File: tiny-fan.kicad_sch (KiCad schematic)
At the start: 41 parts, among them Q1 BSS138, Q2 BSS138, Q3 BSS138, Q4 BSS138, Q5 BSS138, Q6 BSS138, Q7 BSS138, U1 L7812, U2 tiny2040

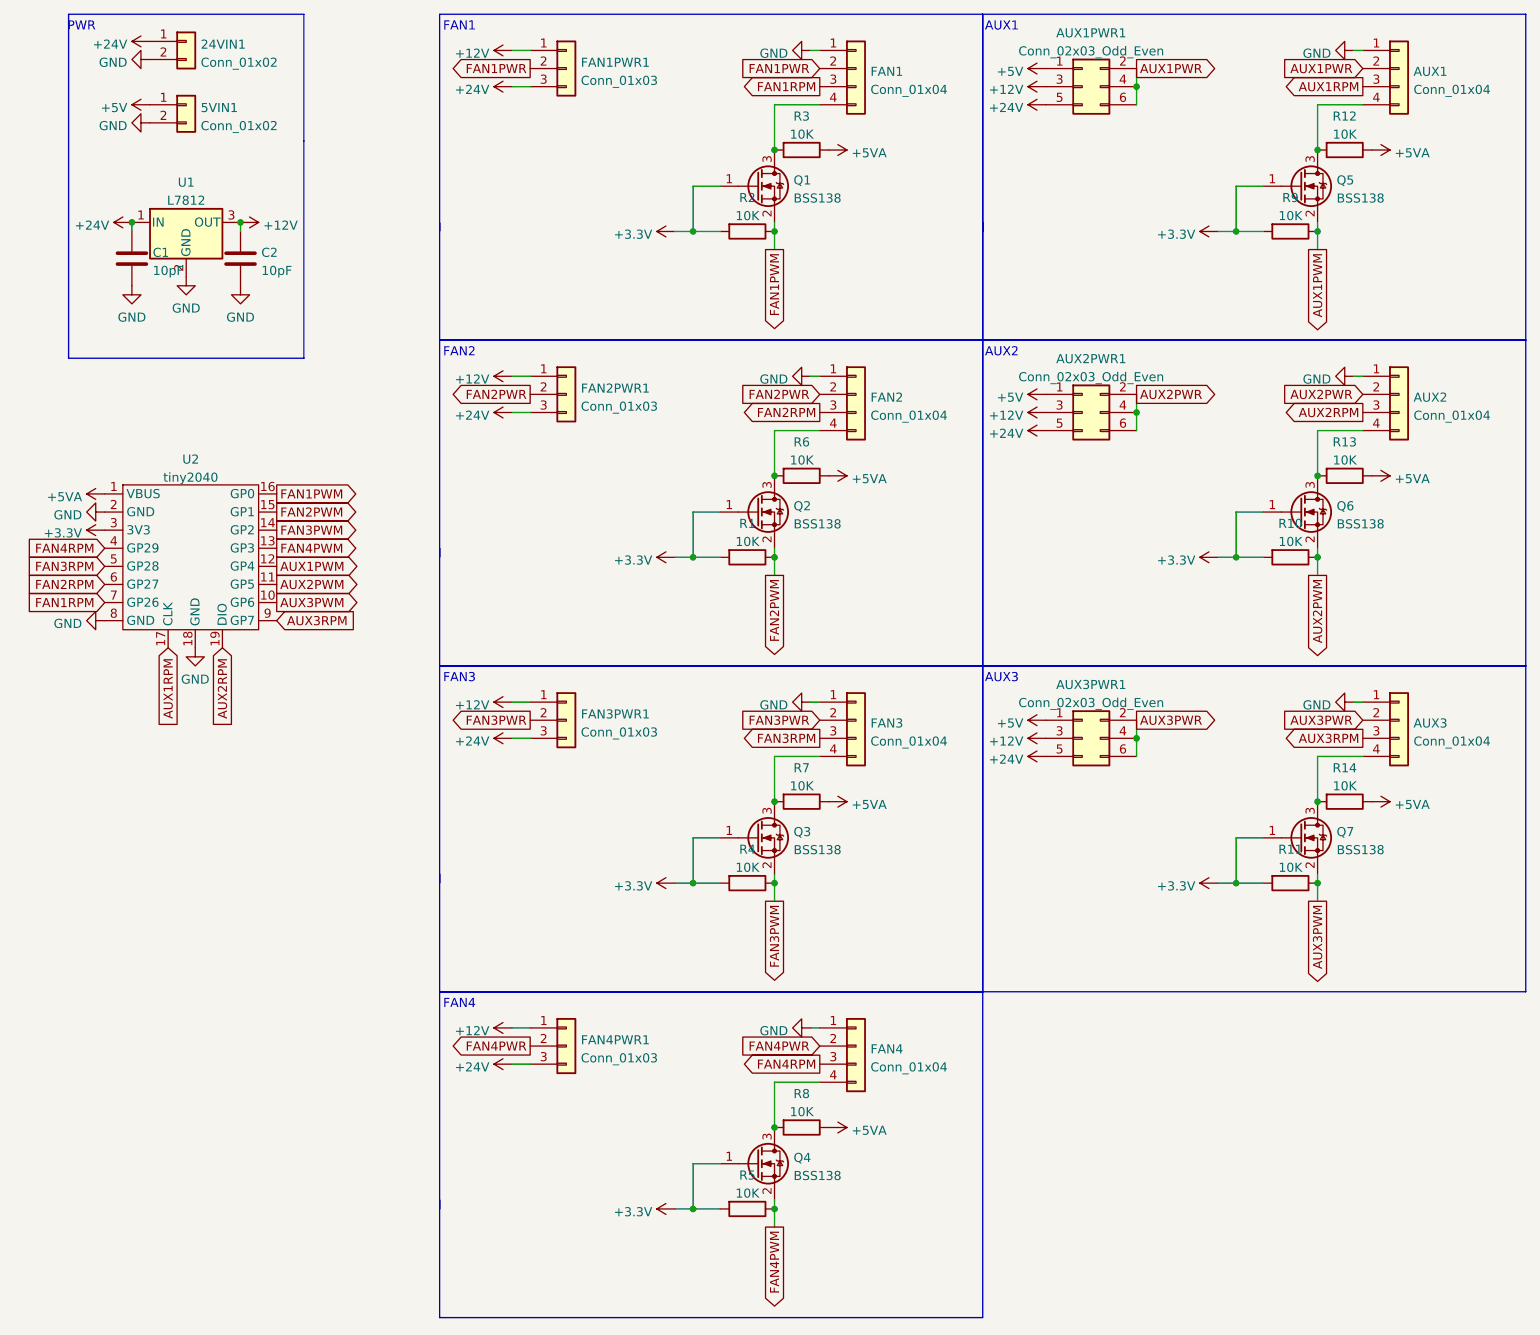
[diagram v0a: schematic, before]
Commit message: version 2
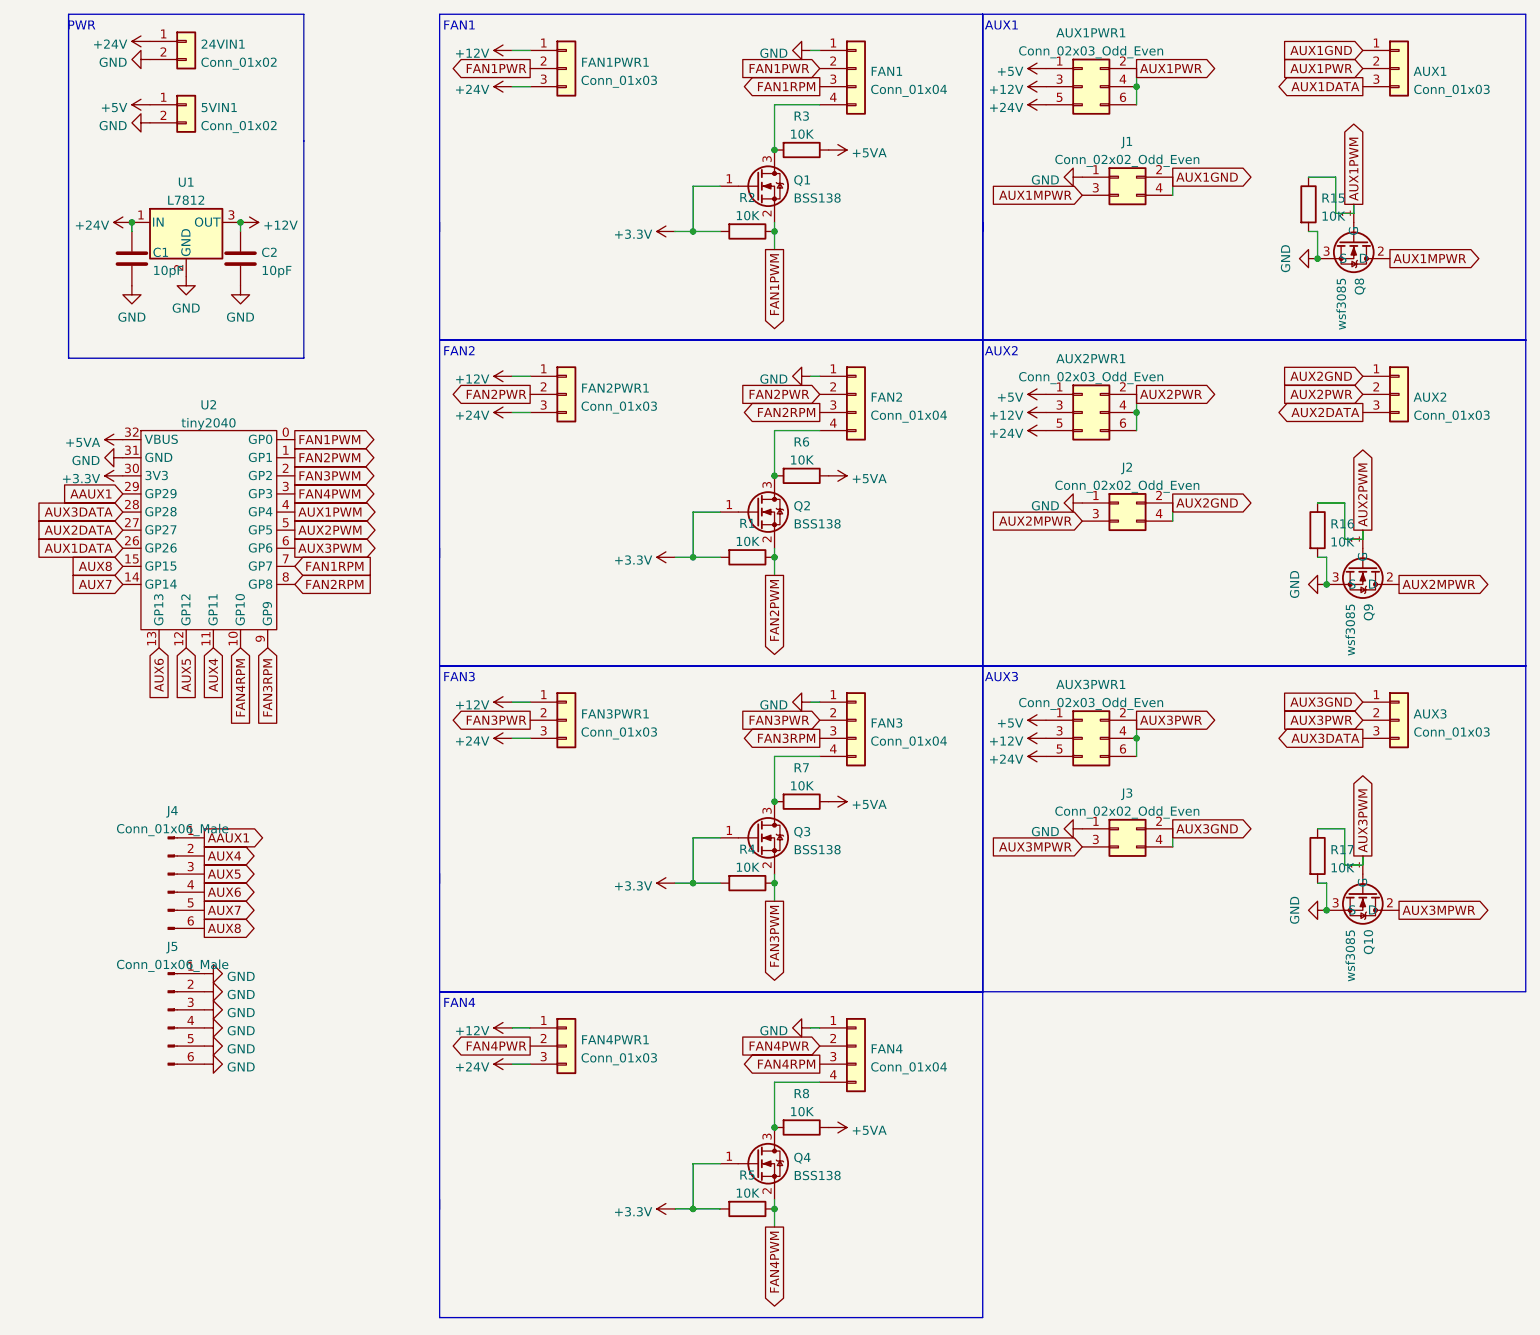
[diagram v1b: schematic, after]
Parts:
- removed Q5, Q6, Q7: BSS138, Package_TO_SOT_SMD:SOT-23, symbol Transistor_FET:BSS138
- removed R10, R11, R12, R13, R14, R9: 10K, Resistor_SMD:R_1206_3216Metric, symbol Device:R
- removed U2: tiny2040, _my_own:tiny2040, symbol tiny2040:tiny2040
- added J1, J2, J3: Conn_02x02_Odd_Even, Connector_PinHeader_2.54mm:PinHeader_2x02_P2.54mm_Vertical, symbol Connector_Generic:Conn_02x02_Odd_Even
- added J4, J5: Conn_01x06_Male, Connector_PinHeader_2.54mm:PinHeader_1x06_P2.54mm_Vertical, symbol Connector:Conn_01x06_Male
- added Q10, Q8, Q9: wsf3085, Package_TO_SOT_SMD:TO-252-2, symbol Transistor_FET:wsf3085
- added R15, R16, R17: 10K, Resistor_SMD:R_1206_3216Metric, symbol Device:R
- added U2: tiny2040, _my_own:rp2040_zero, symbol tiny2040:2040_zero
- AUX1, AUX2, AUX3: value Conn_01x04 -> Conn_01x03; footprint Connector_JST:JST_XH_B4B-XH-AM_1x04_P2.50mm_Vertical -> Connector_JST:JST_XH_B3B-XH-AM_1x03_P2.50mm_Vertical; symbol Connector_Generic:Conn_01x04 -> Connector_Generic:Conn_01x03; LCSC C161871 -> C144394
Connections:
- net +3V3: now also U2.30 (3V3)
- net +5VA: now also U2.32 (VBUS)
- net AUX1PWM: now also Q8.1 (G), R15.1, U2.4 (GP4)
- net AUX2PWM: now also Q9.1 (G), R16.1, U2.5 (GP5)
- net AUX3PWM: now also Q10.1 (G), R17.1, U2.6 (GP6)
- net FAN1PWM: now also U2.0 (GP0)
- net FAN1RPM: now also U2.7 (GP7)
- net FAN2PWM: now also U2.1 (GP1)
- net FAN2RPM: now also U2.8 (GP8)
- net FAN3PWM: now also U2.2 (GP2)
- net FAN3RPM: now also U2.9 (GP9)
- net FAN4PWM: now also U2.3 (GP3)
- net FAN4RPM: now also U2.10 (GP10)
- net GND: now also J1.1 (Pin_1), J2.1 (Pin_1), J3.1 (Pin_1), J5.1 (Pin_1), J5.2 (Pin_2), J5.3 (Pin_3), J5.4 (Pin_4), J5.5 (Pin_5), J5.6 (Pin_6), Q10.3 (S), Q8.3 (S), Q9.3 (S), R15.2, R16.2, R17.2, U2.31 (GND); no longer AUX1.1 (Pin_1), AUX2.1 (Pin_1), AUX3.1 (Pin_1)
- net AUX1RPM renamed AUX1DATA
- net AUX1DATA: now also U2.26 (GP26)
- net AUX2RPM renamed AUX2DATA
- net AUX2DATA: now also U2.27 (GP27)
- net AUX3RPM renamed AUX3DATA
- net AUX3DATA: now also U2.28 (GP28)
- new net AAUX1: J4.1 (Pin_1), U2.29 (GP29)
- new net AUX1GND: AUX1.1 (Pin_1), J1.2 (Pin_2), J1.4 (Pin_4)
- new net AUX1MPWR: J1.3 (Pin_3), Q8.2 (D)
- new net AUX2GND: AUX2.1 (Pin_1), J2.2 (Pin_2), J2.4 (Pin_4)
- new net AUX2MPWR: J2.3 (Pin_3), Q9.2 (D)
- new net AUX3GND: AUX3.1 (Pin_1), J3.2 (Pin_2), J3.4 (Pin_4)
- new net AUX3MPWR: J3.3 (Pin_3), Q10.2 (D)
- new net AUX4: J4.2 (Pin_2), U2.11 (GP11)
- new net AUX5: J4.3 (Pin_3), U2.12 (GP12)
- new net AUX6: J4.4 (Pin_4), U2.13 (GP13)
- new net AUX7: J4.5 (Pin_5), U2.14 (GP14)
- new net AUX8: J4.6 (Pin_6), U2.15 (GP15)
